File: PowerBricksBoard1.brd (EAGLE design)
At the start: 76.2 x 50.8 mm, 16 parts

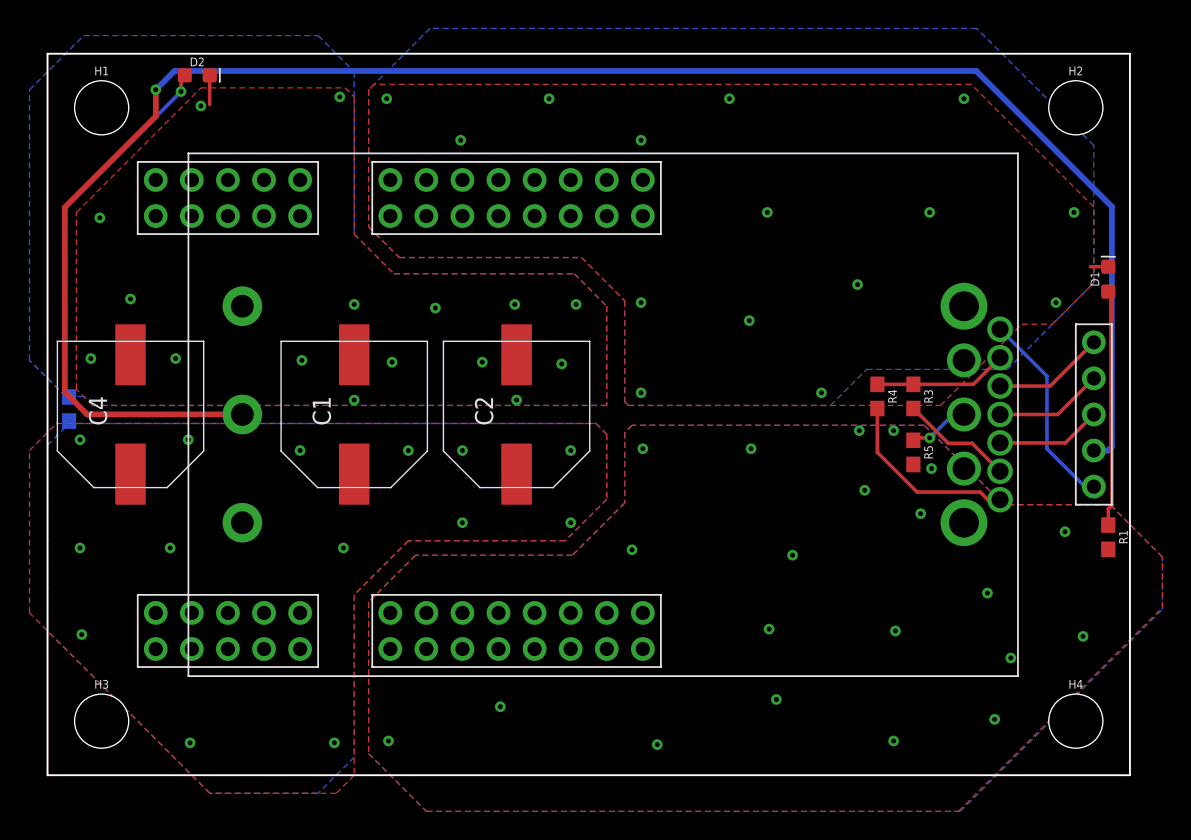
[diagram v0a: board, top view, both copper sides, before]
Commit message: Done but I still need to add a picture Owo
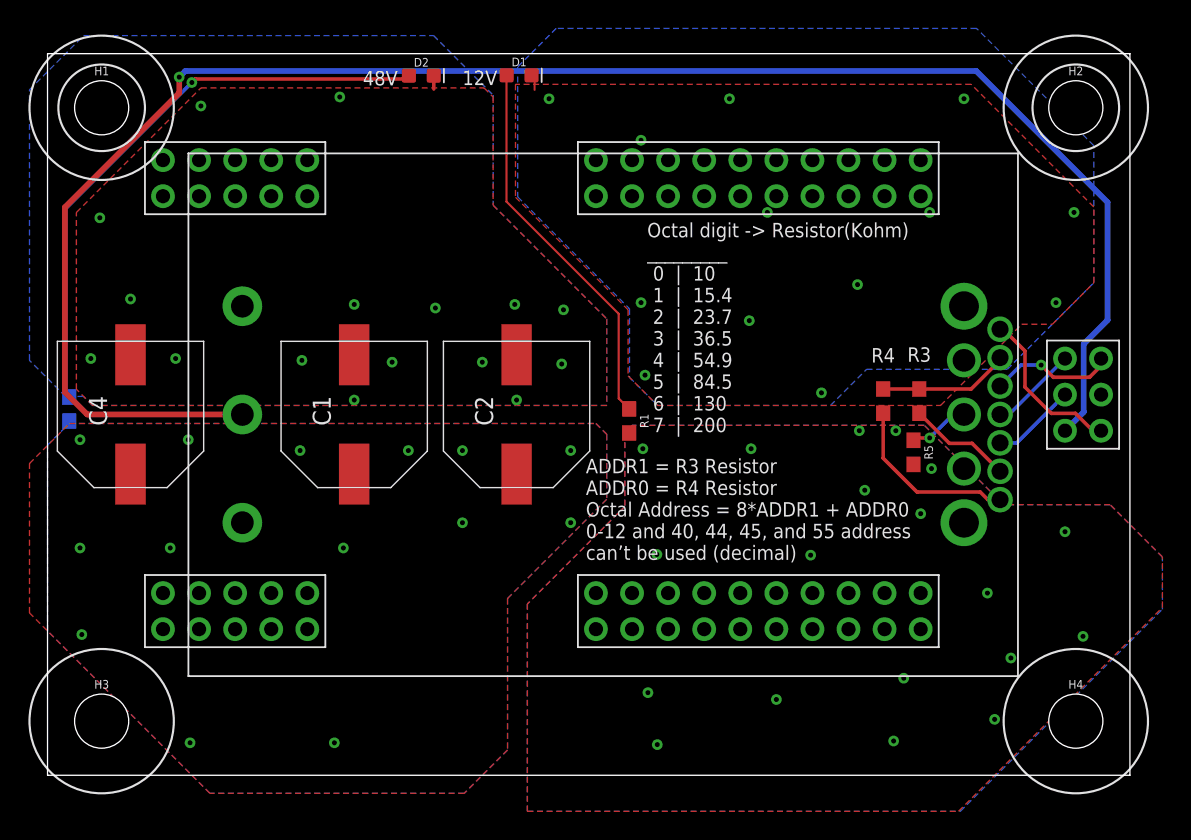
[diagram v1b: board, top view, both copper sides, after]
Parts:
- removed U$3: BRICK2DIST_C, Brick_Dist_Connector:BRICK2DIST_C
- added U$1: BRICK2DIST, Brick_Dist_Connector:BRICK2DIST_D2
- moved D1 43.9 mm to (33.2, 49.3), turned to 0 degrees
- moved R1 34.7 mm to (40.9, 24.9)
- moved D2 15.8 mm to (26.3, 49.3)
- moved R3 0.52 mm to (61.4, 26.3)
- moved R4 0.52 mm to (58.8, 26.3)
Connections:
- net 12V: now also U$1.2@1, U$1.2@10, U$1.2@11, U$1.2@12, U$1.2@13, U$1.2@14, U$1.2@15, U$1.2@16, U$1.2@17, U$1.2@18, U$1.2@19, U$1.2@2, U$1.2@20, U$1.2@3, U$1.2@4, U$1.2@5, U$1.2@6, U$1.2@7, U$1.2@8, U$1.2@9; no longer U$3.2@1, U$3.2@10, U$3.2@11, U$3.2@12, U$3.2@13, U$3.2@14, U$3.2@15, U$3.2@16, U$3.2@2, U$3.2@3, U$3.2@4, U$3.2@5, U$3.2@6, U$3.2@7, U$3.2@8, U$3.2@9
- net 12_GND: now also U$1.4@1, U$1.4@10, U$1.4@11, U$1.4@12, U$1.4@13, U$1.4@14, U$1.4@15, U$1.4@16, U$1.4@17, U$1.4@18, U$1.4@19, U$1.4@2, U$1.4@20, U$1.4@3, U$1.4@4, U$1.4@5, U$1.4@6, U$1.4@7, U$1.4@8, U$1.4@9; no longer U$3.4@1, U$3.4@10, U$3.4@11, U$3.4@12, U$3.4@13, U$3.4@14, U$3.4@15, U$3.4@16, U$3.4@2, U$3.4@3, U$3.4@4, U$3.4@5, U$3.4@6, U$3.4@7, U$3.4@8, U$3.4@9
- net 48V: now also U$1.1@1, U$1.1@10, U$1.1@2, U$1.1@3, U$1.1@4, U$1.1@5, U$1.1@6, U$1.1@7, U$1.1@8, U$1.1@9; no longer U$3.1@1, U$3.1@10, U$3.1@2, U$3.1@3, U$3.1@4, U$3.1@5, U$3.1@6, U$3.1@7, U$3.1@8, U$3.1@9
- net 48_GND: now also U$1.3@1, U$1.3@10, U$1.3@2, U$1.3@3, U$1.3@4, U$1.3@5, U$1.3@6, U$1.3@7, U$1.3@8, U$1.3@9; no longer U$3.3@1, U$3.3@10, U$3.3@2, U$3.3@3, U$3.3@4, U$3.3@5, U$3.3@6, U$3.3@7, U$3.3@8, U$3.3@9
- net ALERT: now also U$1.D; no longer U$3.D
- net C2: now also U$1.A; no longer U$3.A
- net CLK: now also U$1.C; no longer U$3.C
- net DATA: now also U$1.E; no longer U$3.E
- net ON/OFF: now also U$1.B; no longer U$3.B
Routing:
- net N$2: track 26.2 -> 41.4 mm
- net N$1: track 16.6 -> 27.1 mm
- net C2: track 14.2 -> 11.6 mm
- net ON/OFF: track 127.2 -> 125.3 mm
- net ALERT: track 7.66 -> 6.20 mm
- net CLK: track 7.43 -> 5.98 mm
- net 48_GND: track 2.04 -> 0.94 mm
- net DATA: track 7.88 -> 8.93 mm, vias 0 -> 1
- net N$3: track 7.93 -> 7.38 mm
- net 12_GND: track 1.26 -> 1.11 mm, vias 15 -> 13
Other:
- board text added: "12V"
- board text added: "48V"
- board text added: "ADDR1 = R3 Resistor ADDR0 = R4 Resistor Octal Address = 8*ADDR1 + ADDR0 0-12 and 40, 44, 45, and 55 address can’t be used (decimal)"
- board text added: "Octal digit -> Resistor(Kohm) _________ 0 | 10 1 | 15.4 2 | 23.7 3 | 36.5 4 | 54.9 5 | 84.5 6 | 130 7 | 200"
